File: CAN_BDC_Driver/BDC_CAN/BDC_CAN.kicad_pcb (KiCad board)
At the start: 2 copper layers, 87 x 91.6 mm, 56 parts, among them J1 VCC_IN, J2 Motor1_Out, J3 Motor2_Out, J4 CAN, J5 USB_C_Receptacle_USB2.0_16P, J6 Conn_01x05_Pin, Q1 PMOS, Q2 NMOS, Q3 PMOS, Q4 NMOS, Q5 PMOS, Q6 NMOS, Q7 PMOS, Q8 NMOS, SW1 SW_Push, SW2 SW_DIP_x06, U1 STM32F103C8T6, U2 AMS1117, U3 MCP2561-E-MF, U4 TC4427xOA, U5 L7805, U6 TC4427xOA, Y1 Crystal

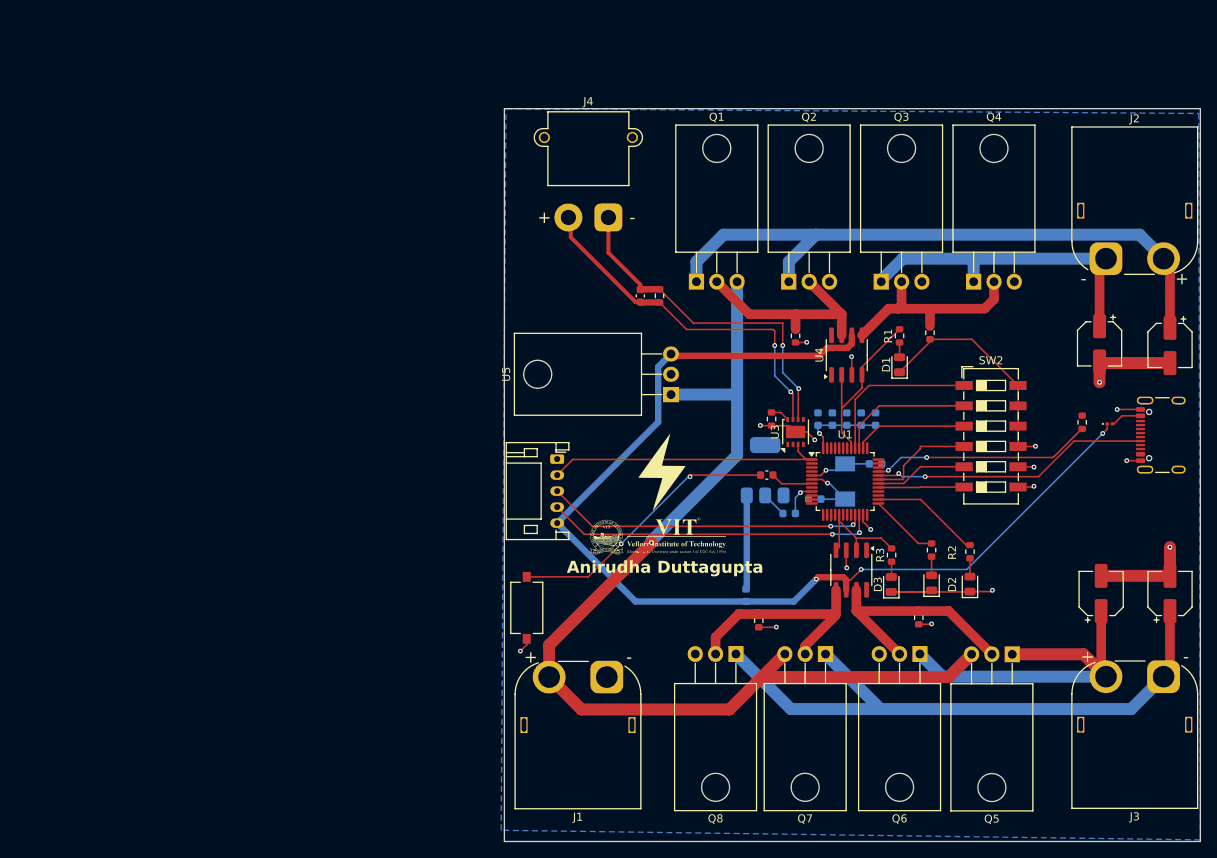
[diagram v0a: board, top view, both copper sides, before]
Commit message: Placement Changed
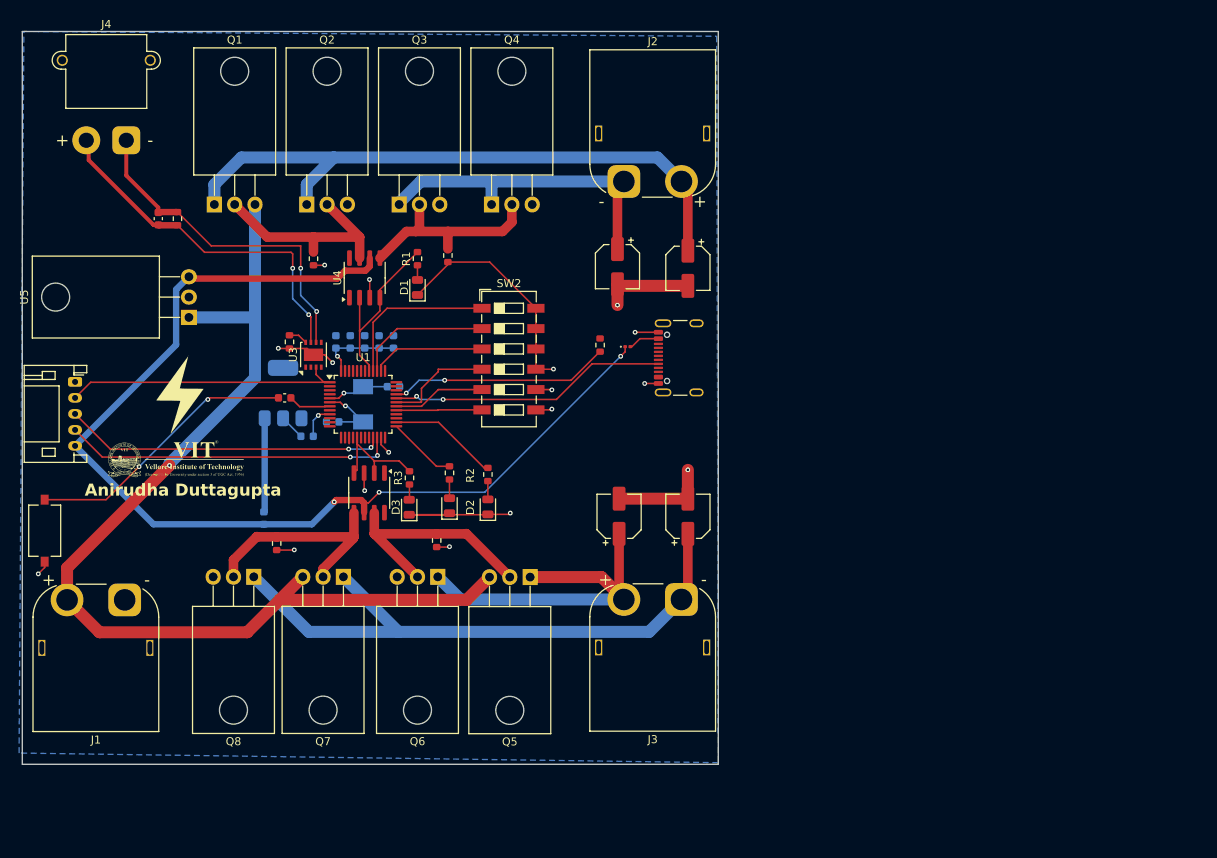
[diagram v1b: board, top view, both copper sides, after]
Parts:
- moved C11 61.0 mm to (85.5, 35.8)
- moved C15 61.0 mm to (143.1, 73.0)
- moved C5 61.0 mm to (109.5, 51.1)
- moved J4 61.0 mm to (81.5, 25.9)
- moved Q2 61.0 mm to (104.1, 34.0)
- moved Q5 61.0 mm to (132.0, 80.5)
- moved R4 61.0 mm to (140.8, 51.5)
- moved C1 61.0 mm to (114.9, 56.8)
- moved C10 61.0 mm to (104.1, 63.0)
- moved C3 61.0 mm to (107.7, 51.1)
- moved C7 61.0 mm to (113.1, 51.1)
- moved C9 61.0 mm to (98.7, 73.2)
- moved D2 61.0 mm to (126.7, 71.8)
- moved D5 61.0 mm to (121.9, 71.6)
- moved G*** 61.0 mm to (88.3, 57.8)
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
